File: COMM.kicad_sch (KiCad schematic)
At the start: 14 parts, among them J1 SMA Conn. (RFPC-SMA30-F), SW1 Inhibit Switch (SS5GLD2), U1 XBee Module (XBP9B-DMSTB002)

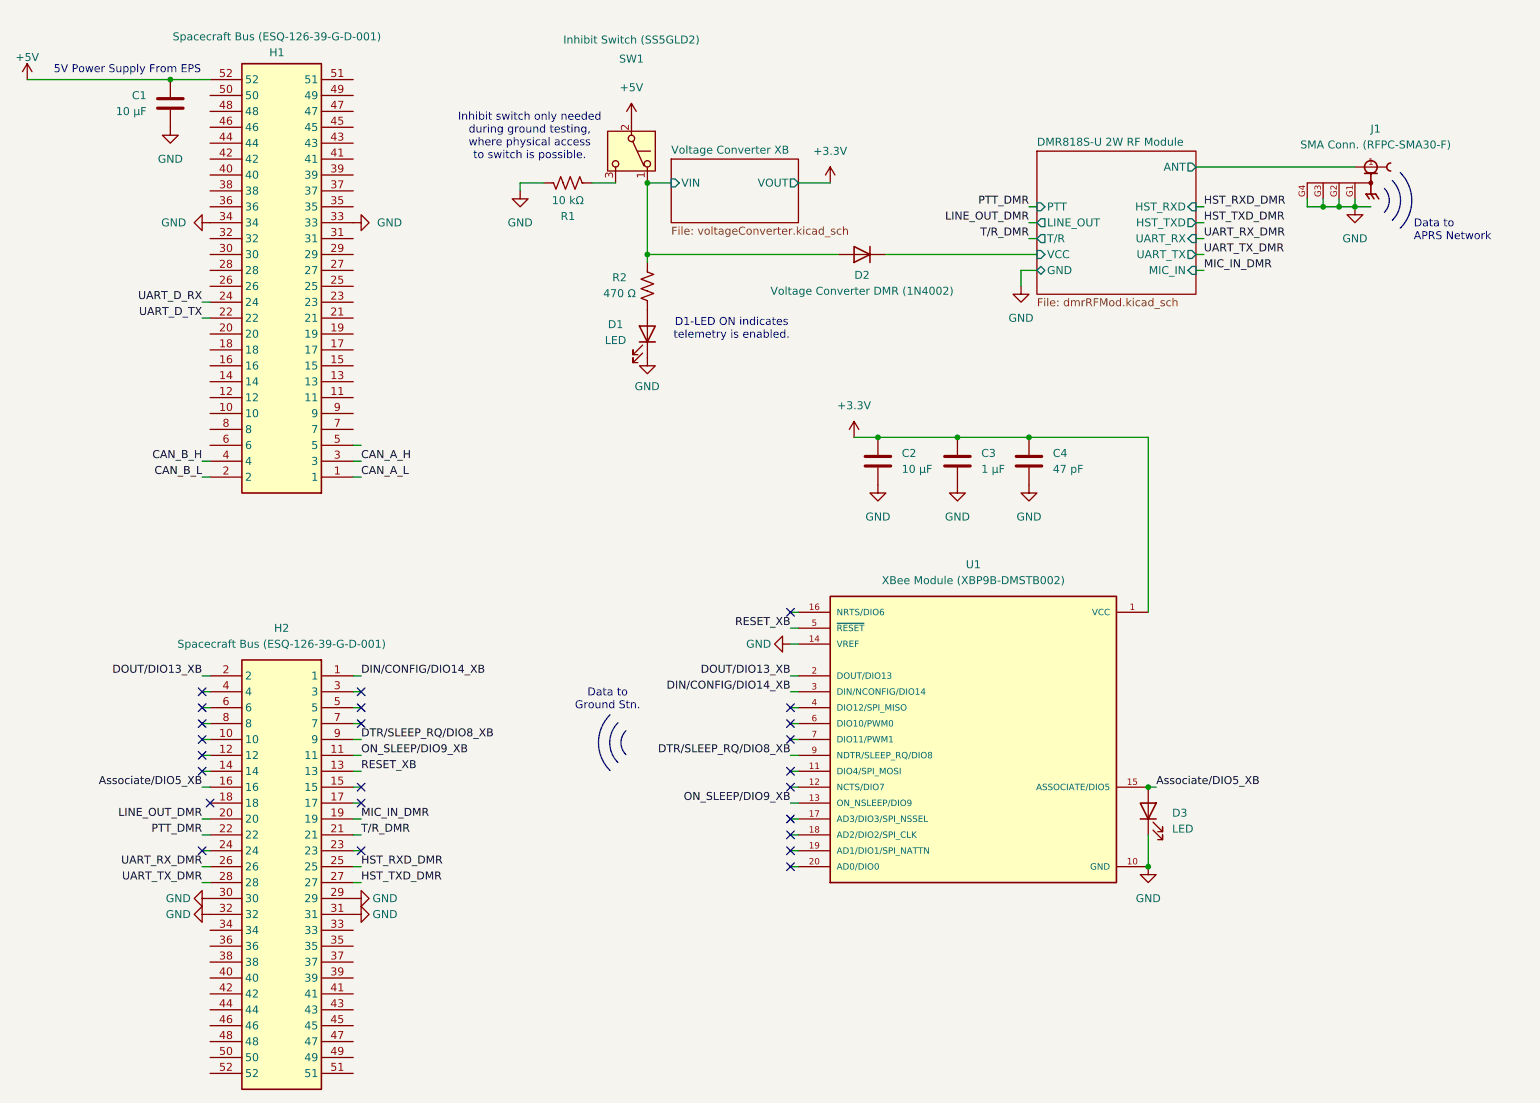
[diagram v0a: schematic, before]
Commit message: Addressed most comments from McPherson, modified schematic.
Signed-off-by: Logan Tolbert <xem6df@virginia.edu>
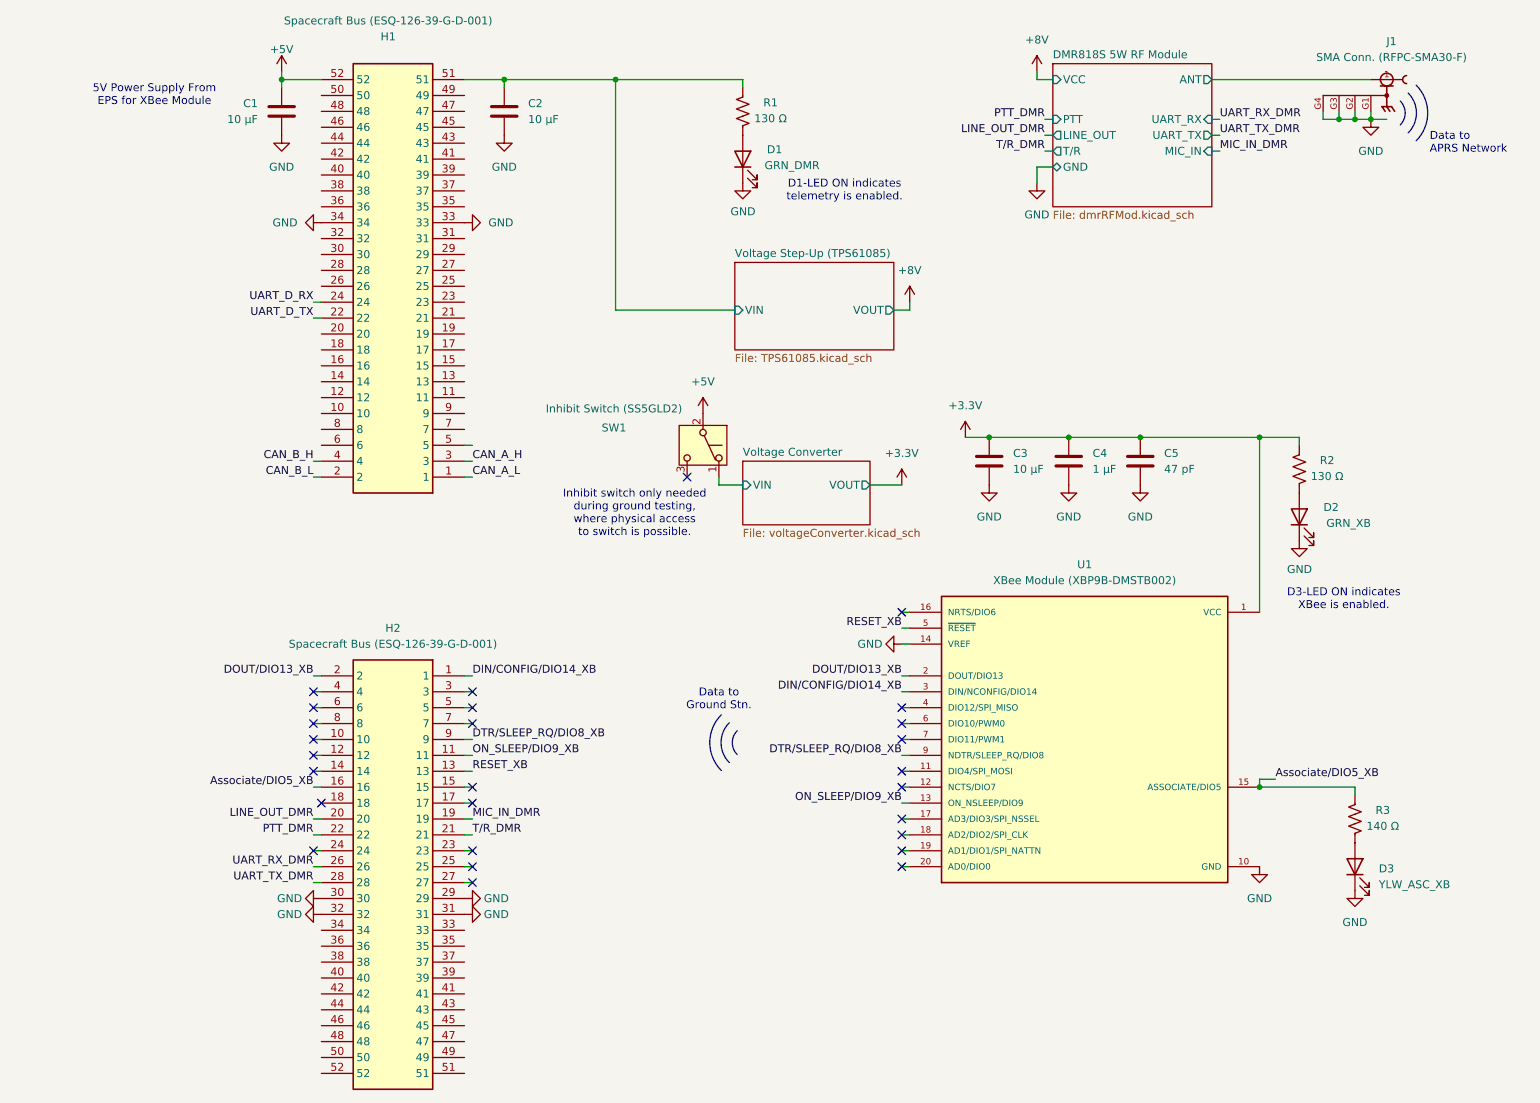
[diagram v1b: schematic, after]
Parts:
- removed D2: Voltage Converter DMR (1N4002), Diode_THT:D_DO-41_SOD81_P10.16mm_Horizontal, symbol Diode:1N4002
- added C2: 10 μF, C_10uF:CAPC1005X70N, symbol Device:C
- added D1: GRN_DMR, LED_THT:LED_D5.0mm, symbol Device:LED
- added R3: 140 Ω, R_470O:RESC6332X65N, symbol Device:R_US
- D2: renamed from D1; value LED -> GRN_XB
- D3: value LED -> YLW_ASC_XB
- R1: value 10 kΩ -> 130 Ω; footprint R_10kO:RESC1005X40N -> R_470O:RESC6332X65N
- R2: value 470 Ω -> 130 Ω
- renumbered C2 to C3, C3 to C4, C4 to C5
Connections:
- net +3.3V: now also R2.2
- net Associate/DIO5_XB: now also R3.2; no longer D3.2 (A)
- net GND: now also C2.2, D1.1 (K); no longer R1.1
- net Voltage Converter/VIN: no longer R2.2
- net at SW1.3 (C): no longer R1.2
- net Voltage Step-Up (TPS61085)/VIN: now reaches H1.51
- net Voltage Step-Up (TPS61085)/VIN: now also R1.2, C2.1
- net HST_RXD_DMR: no longer names the net of H2.25
- net HST_TXD_DMR: no longer names the net of H2.27
- new net: D1.2 (A), R1.1
- new net: D3.2 (A), R3.1
- no-connect marks 24 -> 27
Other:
- sheet DMR818S-U 2W RF Module renamed DMR818S 5W RF Module
- sheet Voltage Converter XB renamed Voltage Converter
- added sheet Voltage Step-Up (TPS61085) (TPS61085.kicad_sch)
- sheet DMR818S 5W RF Module ports: added none; removed HST_RXD, HST_TXD
- note added: "5V Power Supply From EPS for XBee Module"
- note added: "D3-LED ON indicates XBee is enabled."
- note removed: "5V Power Supply From EPS"
- moved on the sheet: C1, C3, C4, C5, D2, D3, H1, H2, J1, R2, SW1, U1
